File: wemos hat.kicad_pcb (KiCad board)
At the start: 2 copper layers, 16 parts, among them J1 RJ45, U1 MAX3072E, U2 WeMos_mini

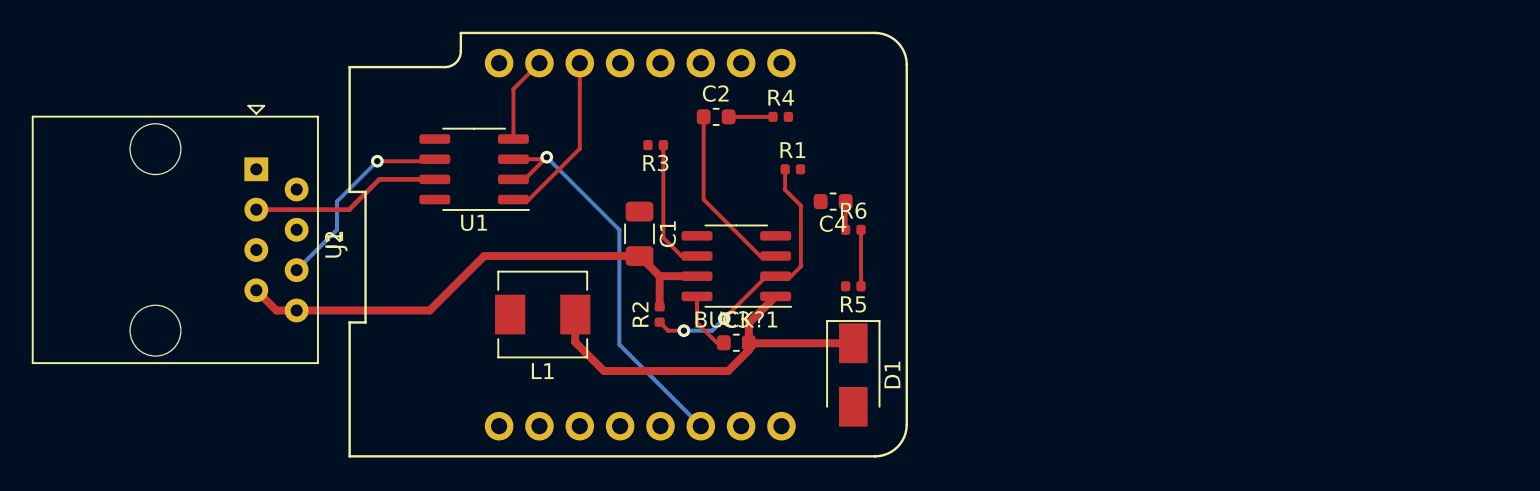
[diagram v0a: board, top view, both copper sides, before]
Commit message: Components done
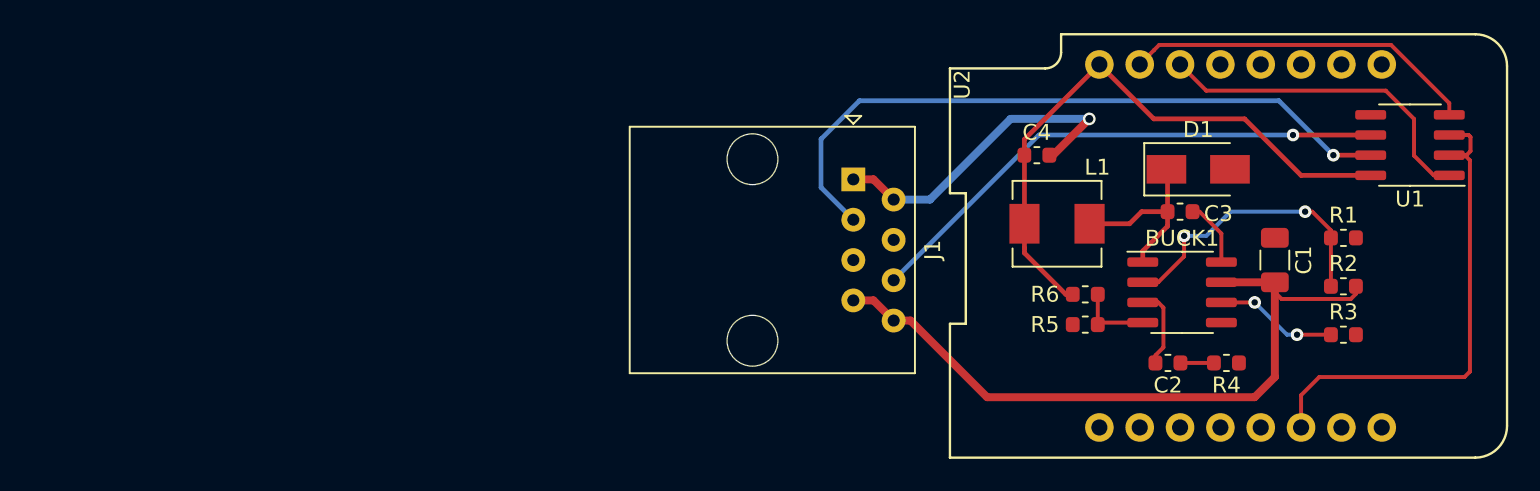
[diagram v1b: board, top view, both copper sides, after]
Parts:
- R1, R2, R3, R4, R5, R6: footprint Resistor_SMD:R_0402_1005Metric -> Resistor_SMD:R_0603_1608Metric
- moved U1 58.9 mm to (168.7, 79.0)
- moved R3 44.9 mm to (164.5, 90.9), turned to 0 degrees
- moved R2 43.1 mm to (164.5, 87.9), turned to 0 degrees
- moved C1 40.0 mm to (160.1, 86.2)
- moved U2 37.8 mm to (158.0, 85.3)
- moved J1 37.6 mm to (133.6, 81.2)
- moved R1 34.9 mm to (164.5, 84.8)
- moved L1 32.9 mm to (146.4, 83.9)
- moved C2 32.4 mm to (153.4, 92.7)
- moved R4 32.1 mm to (157.1, 92.7)
- moved C3 29.1 mm to (154.2, 83.2), turned to 180 degrees
- moved BUCK1 28.1 mm to (154.3, 88.3), turned to 0 degrees
- moved D1 25.3 mm to (155.3, 80.5), turned to 0 degrees
- moved R6 15.2 mm to (148.2, 88.4)
- moved R5 14.8 mm to (148.2, 90.3)
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- renumbered BUCK?1 to BUCK1
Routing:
- net VCC: track 1.78 -> 37.9 mm
- net Net-(J1-Pad3): track 12.0 -> 43.0 mm, vias 0 -> 1
- net Net-(J1-Pad6): track 12.6 -> 33.8 mm
- net GND: track 0.00 -> 21.0 mm, vias 0 -> 1
- net Net-(U1-Pad4): track 5.46 -> 22.3 mm
- net Net-(BUCK1-Pad7): track 32.2 -> 45.4 mm
- net Net-(BUCK1-Pad1): track 24.7 -> 11.7 mm
- net Net-(U1-Pad1): track 10.9 -> 21.2 mm
- net Net-(BUCK1-Pad3): track 11.2 -> 5.13 mm
- net Net-(U1-Pad2): track 25.8 -> 31.7 mm, vias 1 -> 0
- net Net-(BUCK1-Pad4): track 3.56 -> 4.79 mm
- net Net-(BUCK1-Pad2): track 17.3 -> 18.5 mm
- net Net-(BUCK1-Pad6): track 8.43 -> 7.74 mm, vias 0 -> 2
- net Net-(C2-Pad2): track 2.79 -> 2.11 mm
